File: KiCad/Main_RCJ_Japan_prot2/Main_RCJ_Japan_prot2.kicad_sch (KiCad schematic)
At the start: 21 parts, among them J1 Conn_01x04_Socket, J2 Conn_01x04_Socket, J3 Conn_01x04_Socket, J4 Conn_01x04_Socket, J5 Conn_01x04_Socket, J6 Conn_01x04_Socket, J7 Conn_01x02_Socket, J8 Conn_01x06_Socket, J9 Conn_02x05_Counter_Clockwise, SW1 SW_Push

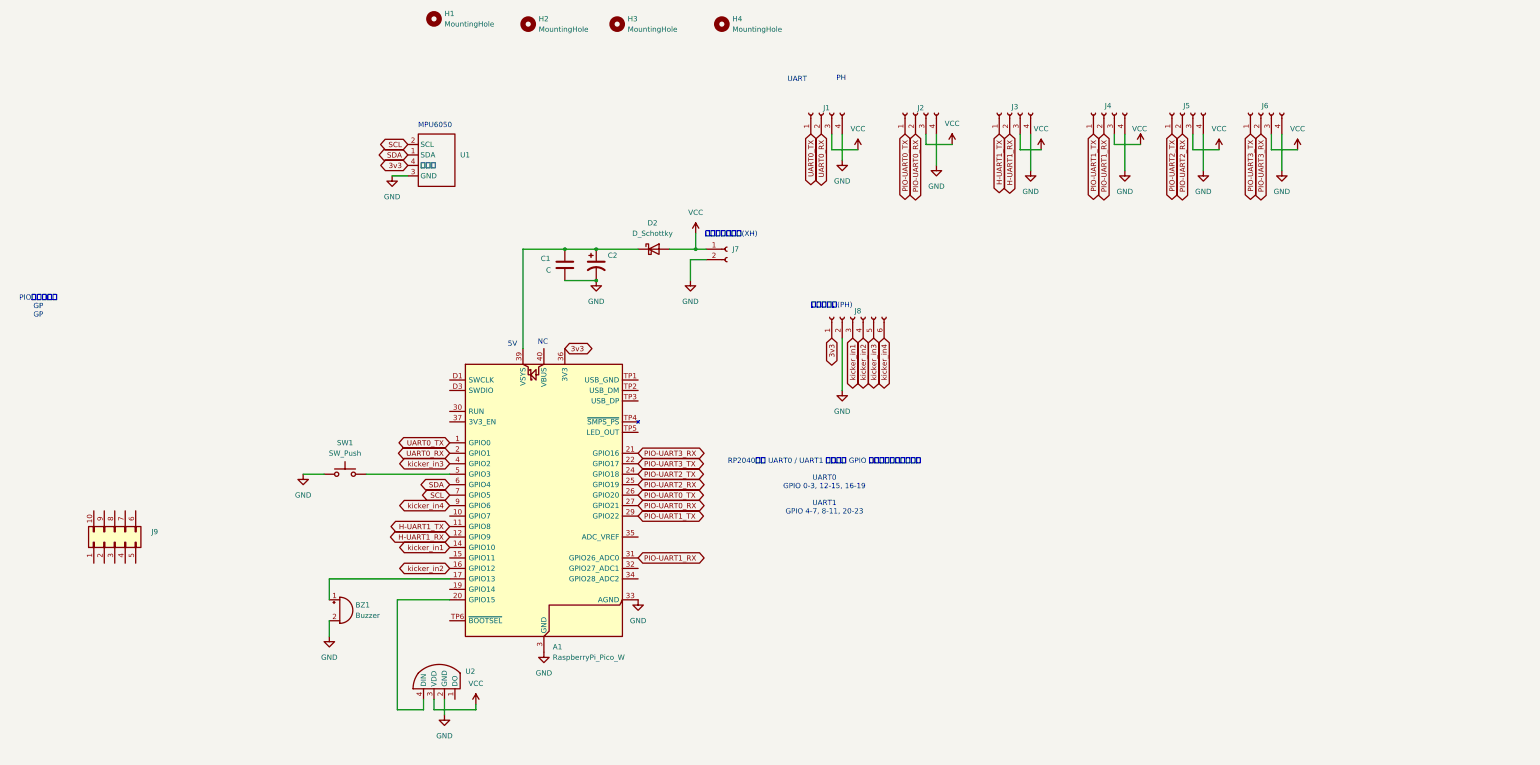
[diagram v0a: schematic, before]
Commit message: 新メイン完成
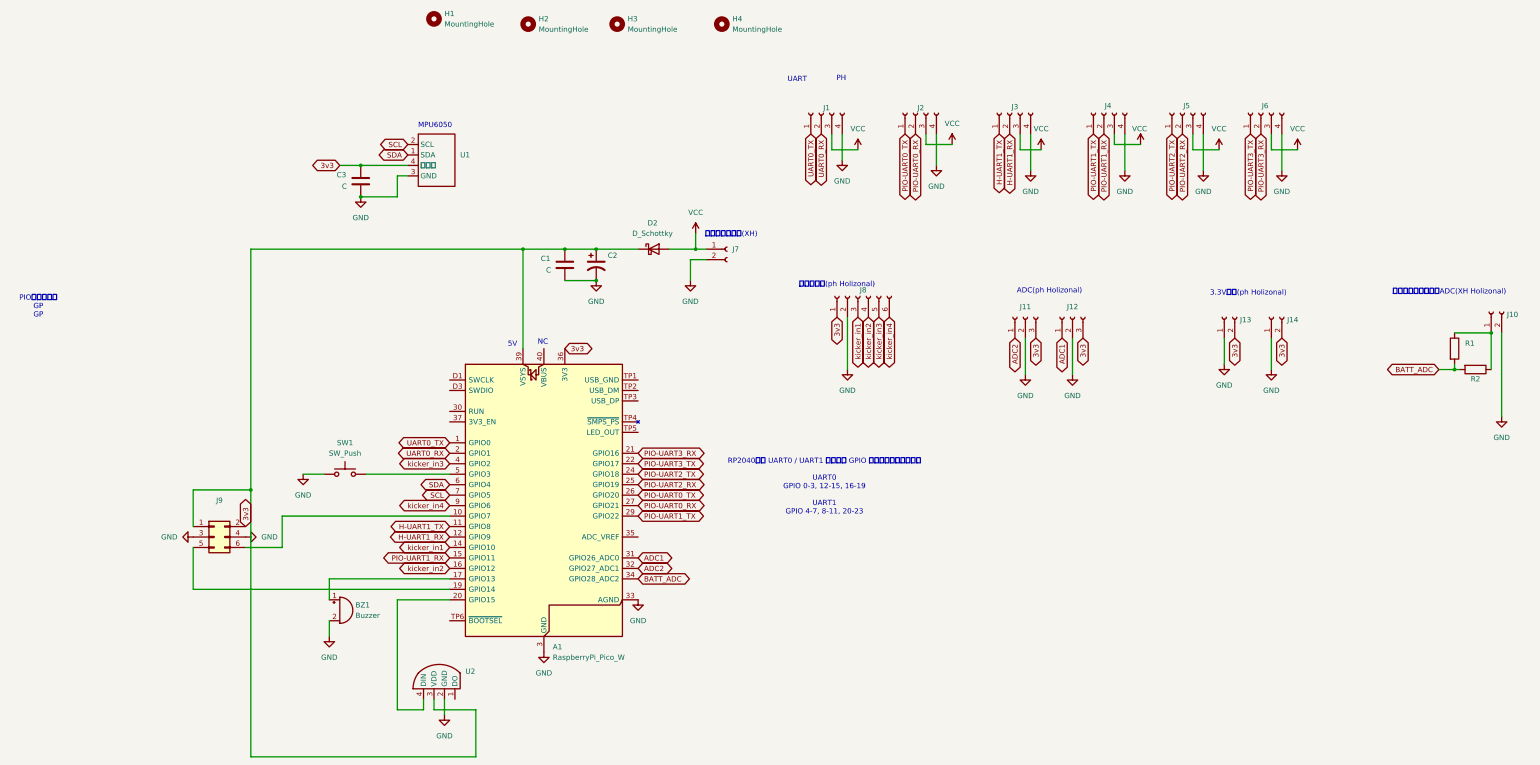
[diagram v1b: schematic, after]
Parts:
- removed J9: Conn_02x05_Counter_Clockwise, symbol Connector_Generic:Conn_02x05_Counter_Clockwise
- added C3: C, Capacitor_SMD:C_0603_1608Metric_Pad1.08x0.95mm_HandSolder, symbol Device:C
- added J10: Conn_01x02_Socket, Connector_JST:JST_XH_S2B-XH-A_1x02_P2.50mm_Horizontal, symbol Connector:Conn_01x02_Socket
- added J11, J12: Conn_01x03_Socket, Connector_JST:JST_PH_B3B-PH-K_1x03_P2.00mm_Vertical, symbol Connector:Conn_01x03_Socket
- added J13, J14: Conn_01x02_Socket, Connector_JST:JST_PH_B2B-PH-K_1x02_P2.00mm_Vertical, symbol Connector:Conn_01x02_Socket
- added J9: Conn_02x03_Odd_Even, Connector_PinHeader_2.54mm:PinHeader_2x03_P2.54mm_Vertical, symbol Connector_Generic:Conn_02x03_Odd_Even
- added R1, R2: R, Resistor_THT:R_Axial_DIN0309_L9.0mm_D3.2mm_P12.70mm_Horizontal, symbol Device:R
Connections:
- net 3v3: now also C3.1, J11.3 (Pin_3), J12.3 (Pin_3), J13.2 (Pin_2), J14.2 (Pin_2), J9.2 (Pin_2)
- net GND: now also C3.2, J10.2 (Pin_2), J11.2 (Pin_2), J12.2 (Pin_2), J13.1 (Pin_1), J14.1 (Pin_1), J9.3 (Pin_3), J9.4 (Pin_4)
- net PIO-UART1_RX: now also A1.15 (GPIO11); no longer A1.31 (GPIO26_ADC0)
- net VCC: no longer U2.3 (VDD)
- net at A1.39 (VSYS), C1.1, C2.1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: now also U2.3 (VDD), J9.1 (Pin_1)
- net at A1.10 (GPIO7): now also J9.6 (Pin_6)
- net at A1.19 (GPIO14): now also J9.5 (Pin_5)
- net ADC2: now reaches A1.32 (GPIO27_ADC1)
- net ADC2: now also J11.1 (Pin_1)
- net BATT_ADC: now reaches A1.34 (GPIO28_ADC2)
- net BATT_ADC: now also R1.2, R2.2
- new net: J10.1 (Pin_1), R1.1, R2.1
- new net ADC1: A1.31 (GPIO26_ADC0), J12.1 (Pin_1)
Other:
- note added: "3.3V供給(ph Holizonal)"
- note added: "ADC(ph Holizonal)"
- note added: "キッカー用(ph Holizonal)"
- note added: "バッテリー電圧測定ADC(XH Holizonal)"
- note removed: "キッカー用(PH)"
- moved on the sheet: J8
